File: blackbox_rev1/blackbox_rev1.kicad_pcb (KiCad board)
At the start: 2 copper layers, 16 parts, among them J1 RJ45_LED_Shielded, J2 Molex_uF_SV_06, SW1 SW_Push, SW2 SW_Push, U1 Teensy4.1_DEV-16771, U2 TSR1-2433

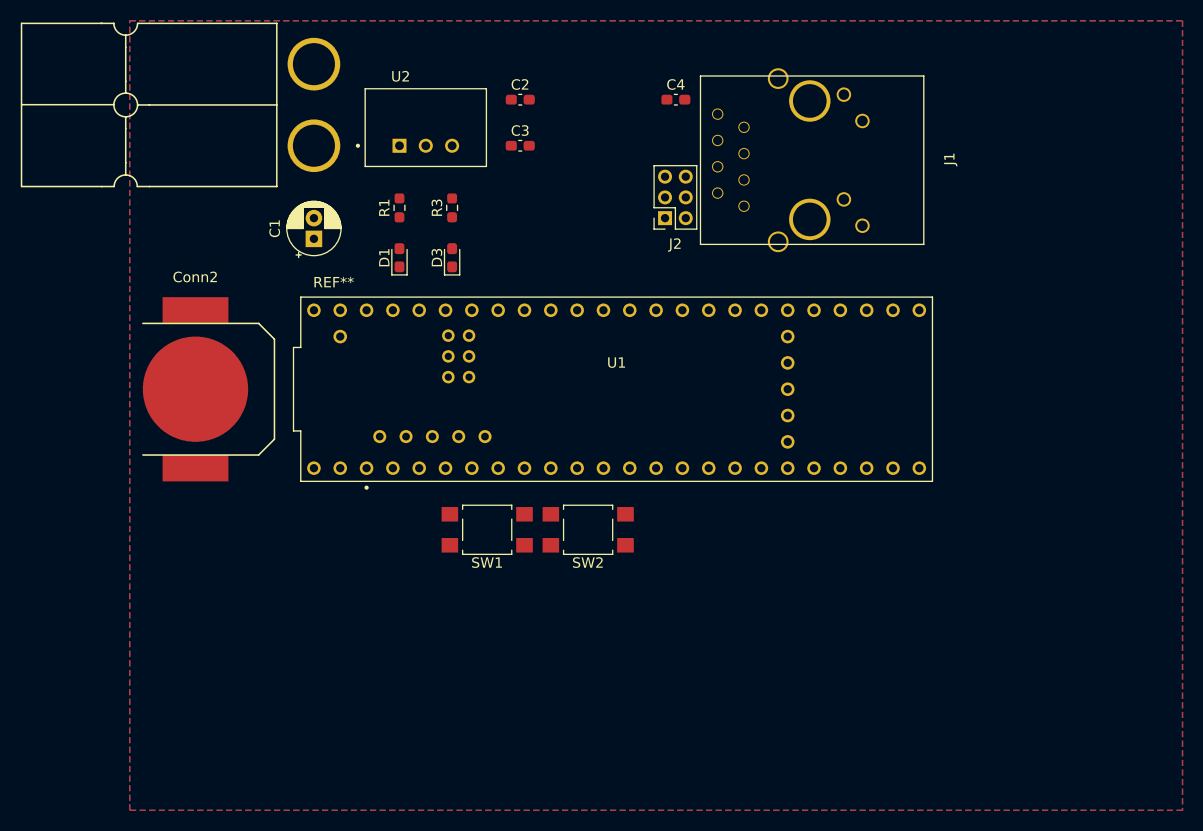
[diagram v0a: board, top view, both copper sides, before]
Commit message: finish layout design
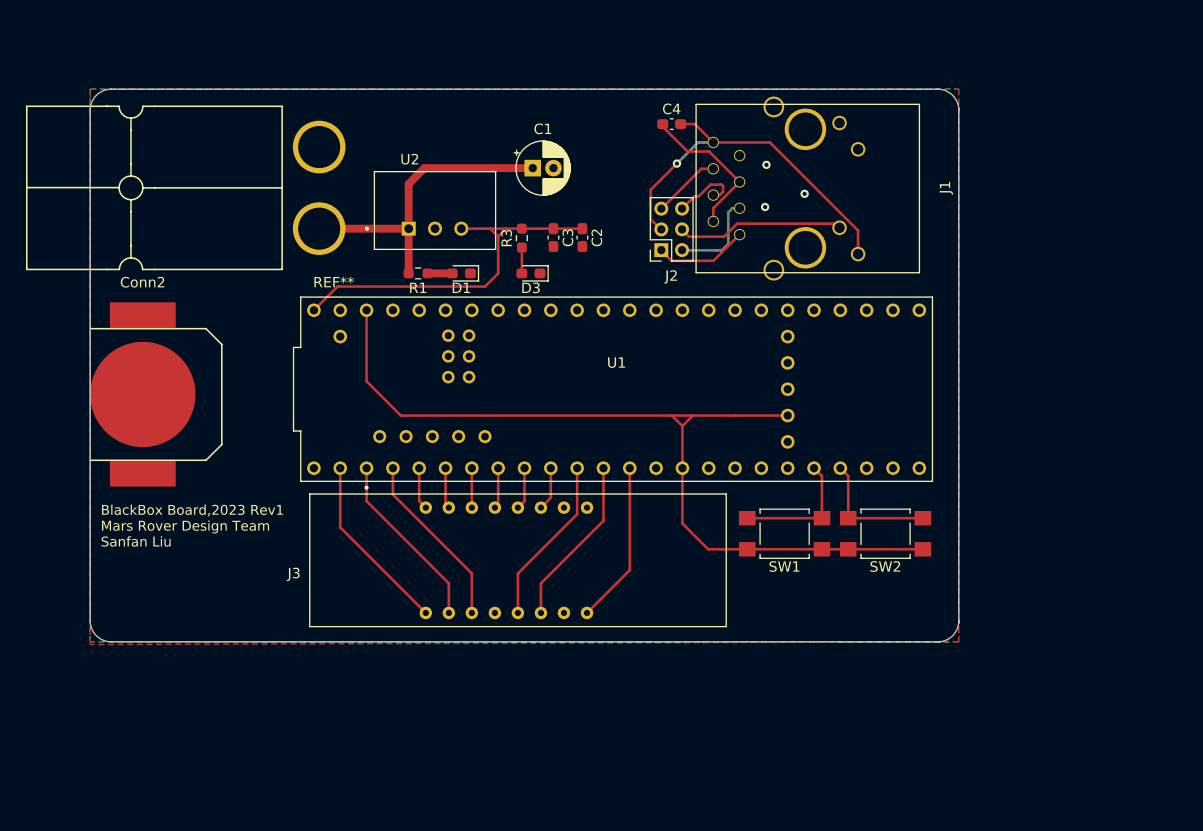
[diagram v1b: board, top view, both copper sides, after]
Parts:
- added J3: Conn_02x08_Counter_Clockwise, blackbox_rev1:timerLED, F.Cu at (89.5, 92.7)
- moved SW1 28.7 mm to (124.2, 95.2)
- moved SW2 28.7 mm to (133.9, 95.2)
- moved C1 22.2 mm to (99.9, 59.9), turned to 0 degrees
- moved C2 14.6 mm to (104.6, 66.6), turned to -90 degrees
- moved C3 9.42 mm to (101.9, 66.6), turned to -90 degrees
- moved U2 8.05 mm to (90.4, 64.0)
- moved Conn1 8.02 mm to (79.2, 57.9)
- moved D3 7.75 mm to (99.7, 70.1), turned to 180 degrees
- moved R3 7.34 mm to (98.8, 66.7)
- moved R1 6.58 mm to (88.8, 70.1), turned to 180 degrees
- moved D1 6.16 mm to (93.0, 70.1), turned to 180 degrees
- moved Conn2 5.11 mm to (62.2, 74.2)
- moved J2 3.11 mm to (112.3, 67.9)
- moved J1 2.77 mm to (139.2, 61.8)
- moved C4 2.39 mm to (113.3, 55.7)
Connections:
- C2 pad 1: +3V3 -> +5V
- C3 pad 1: +3V3 -> +5V
- R3 pad 2: +3V3 -> +5V
- U1 pad 0: Display_A -> Display_D1_Low
- U1 pad 1: Display_B -> Display_D2_Low
- U1 pad 10: unconnected-(U1-Pad10) -> Display_D3_Low
- U1 pad 11: unconnected-(U1-Pad11) -> Display_D4_Low
- U1 pad 2: Display_C -> Display_D
- U1 pad 24: Display_D1_Low -> unconnected-(U1-Pad24)
- U1 pad 25: Display_D2_Low -> unconnected-(U1-Pad25)
- U1 pad 26: Display_D3_Low -> unconnected-(U1-Pad26)
- U1 pad 27: Display_D4_Low -> unconnected-(U1-Pad27)
- U1 pad 28: unconnected-(U1-Pad28) -> Sw_Hour
- U1 pad 29: unconnected-(U1-Pad29) -> Sw_Min
- U1 pad 3: Display_D -> Display_B
- U1 pad 4: Display_E -> Display_G
- U1 pad 5: Display_F -> Display_A
- U1 pad 6: Display_G -> Display_C
- U1 pad 7: Sw_Hour -> Clock_SquareWave
- U1 pad 8: Sw_Min -> Display_F
- U1 pad 9: unconnected-(U1-Pad9) -> Display_E
- U1 pad VIN: unconnected-(U1-PadVIN) -> +5V
- U2 pad 3: +3V3 -> +5V
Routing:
- net +3V3: track 0.00 -> 85.4 mm
- net +5V: track 0.00 -> 36.6 mm
- net Net-(C4-Pad2): track 0.00 -> 36.1 mm, vias 0 -> 1
- net +36V: track 0.00 -> 29.9 mm
- net Display_D1_Low: track 0.00 -> 17.4 mm
- net Display_D2_Low: track 0.00 -> 17.3 mm
- net Display_D: track 0.00 -> 17.1 mm
- net Display_D3_Low: track 0.00 -> 16.5 mm
- net Display_E: track 0.00 -> 16.3 mm
- net Net-(J1-Pad10): track 0.00 -> 16.2 mm
- net Display_D4_Low: track 0.00 -> 15.7 mm
- net Net-(C4-Pad1): track 0.00 -> 14.9 mm
- net Sw_Min: track 0.00 -> 12.3 mm
- net Sw_Hour: track 0.00 -> 12.3 mm
- net Net-(J1-Pad3): track 0.00 -> 9.81 mm
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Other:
- board outline added: 83.8 x 53.3 mm
- board text added: "BlackBox Board,2023 Rev1 Mars Rover Design Team Sanfan Liu"
